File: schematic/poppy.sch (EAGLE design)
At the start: 18 parts, among them Q1 8MHz

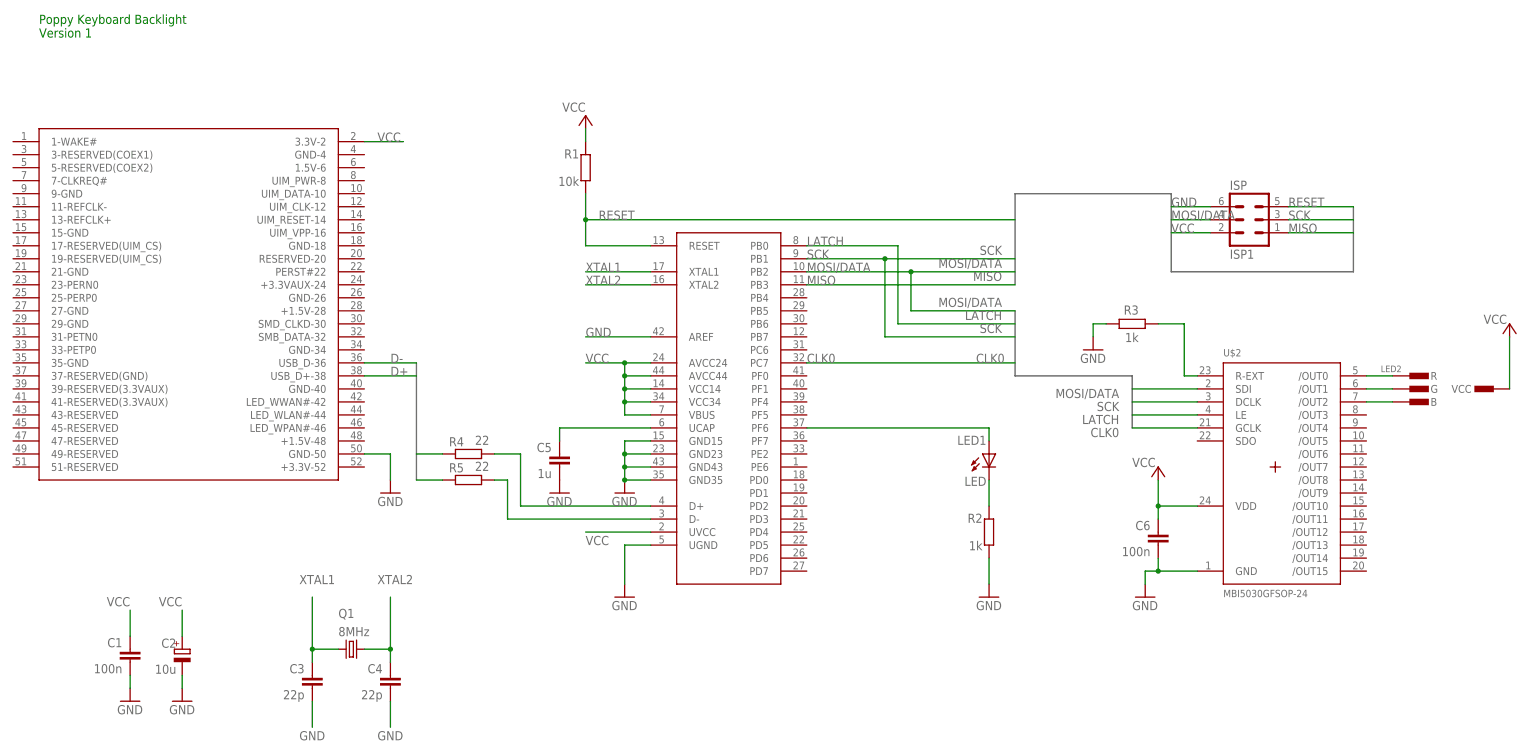
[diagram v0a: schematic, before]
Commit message: routed everything
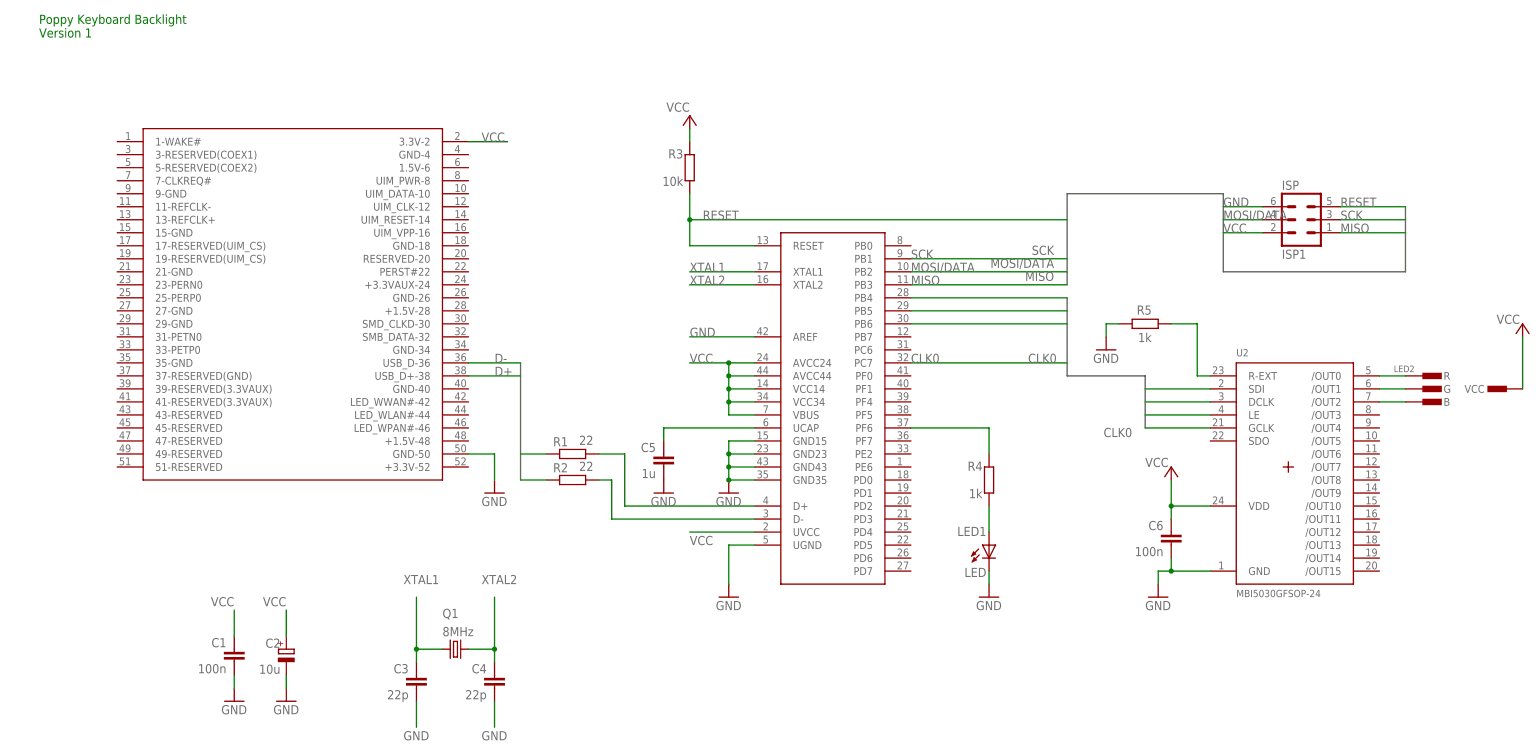
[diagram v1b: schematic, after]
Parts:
- removed U$1: ATMEGA16U4TQFP44, p1poppy:ATMEGA16U4TQFP44
- removed U$2: MBI5030GFSOP-24, p1poppy:MBI5030GFSOP-24
- added U1: ATMEGA16U4TQFP44, p1poppy:ATMEGA16U4TQFP44
- added U2: MBI5030GFSOP-24, p1poppy:MBI5030GFSOP-24
- R1: value 10k -> 22; device resistor:R-EU_R3216 -> resistor:R-EU_R1206
- R2: value 1k -> 22; device resistor:R-EU_R3216 -> resistor:R-EU_R1206
- R3: value 1k -> 10k; device resistor:R-EU_R3216 -> resistor:R-EU_R1206
- R4, R5: value 22 -> 1k; device resistor:R-EU_R3216 -> resistor:R-EU_R1206
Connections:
- new net DCLK: U1.PB4, U2.DCLK
- new net SDI: U1.PB5, U2.SDI
- net CLK0: now also U1.PC7, U2.GCLK; no longer U$1.PC7, U$2.GCLK
- net D+: now also R1.2; no longer R4.2
- net D-: now also R2.2; no longer R5.2
- net GND: now also LED1.C, R5.1, U1.AREF, U1.GND15, U1.GND23, U1.GND35, U1.GND43, U1.UGND, U2.GND; no longer R2.1, R3.1, U$1.AREF, U$1.GND15, U$1.GND23, U$1.GND35, U$1.GND43, U$1.UGND, U$2.GND
- net LATCH: now also U1.PB6, U2.LE; no longer U$1.PB0, U$2.LE
- net MISO: now also U1.PB3; no longer U$1.PB3
- net MOSI/DATA: now also U1.PB2; no longer U$1.PB2, U$2.SDI
- net N$1: now also R4.2, U1.PF6; no longer LED1.A, U$1.PF6
- net N$10: now also R2.1, U1.D-; no longer R5.1, U$1.D-
- net N$2: now also R5.2, U2.R-EXT; no longer R3.2, U$2.R-EXT
- net N$3: now also U2./OUT0; no longer U$2./OUT0
- net N$4: now also U1.UCAP; no longer U$1.UCAP
- net N$5: now also U2./OUT1; no longer U$2./OUT1
- net N$6: now also U2./OUT2; no longer U$2./OUT2
- net N$7: now also LED1.A, R4.1; no longer LED1.C, R2.2
- net N$9: now also R1.1, U1.D+; no longer R4.1, U$1.D+
- net RESET: now also R3.1, U1.RESET; no longer R1.1, U$1.RESET
- net SCK: now also U1.PB1; no longer U$1.PB1, U$2.DCLK
- net VCC: now also R3.2, U1.AVCC24, U1.AVCC44, U1.UVCC, U1.VBUS, U1.VCC14, U1.VCC34, U2.VDD; no longer R1.2, U$1.AVCC24, U$1.AVCC44, U$1.UVCC, U$1.VBUS, U$1.VCC14, U$1.VCC34, U$2.VDD
- net XTAL1: now also U1.XTAL1; no longer U$1.XTAL1
- net XTAL2: now also U1.XTAL2; no longer U$1.XTAL2
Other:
- moved on the sheet: C1, C2, C3, C4, C5, C6, ISP, LED1, LED2, Q1, R1, R2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
